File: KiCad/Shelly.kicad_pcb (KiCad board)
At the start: 2 copper layers, 15 x 30 mm, 15 parts, among them J1 Shelly 1, J2 Shelly 2, J3 Shelly i3, J4 USB-C, U1 FT231XQ, U2 G3VM-61VY3(TR)

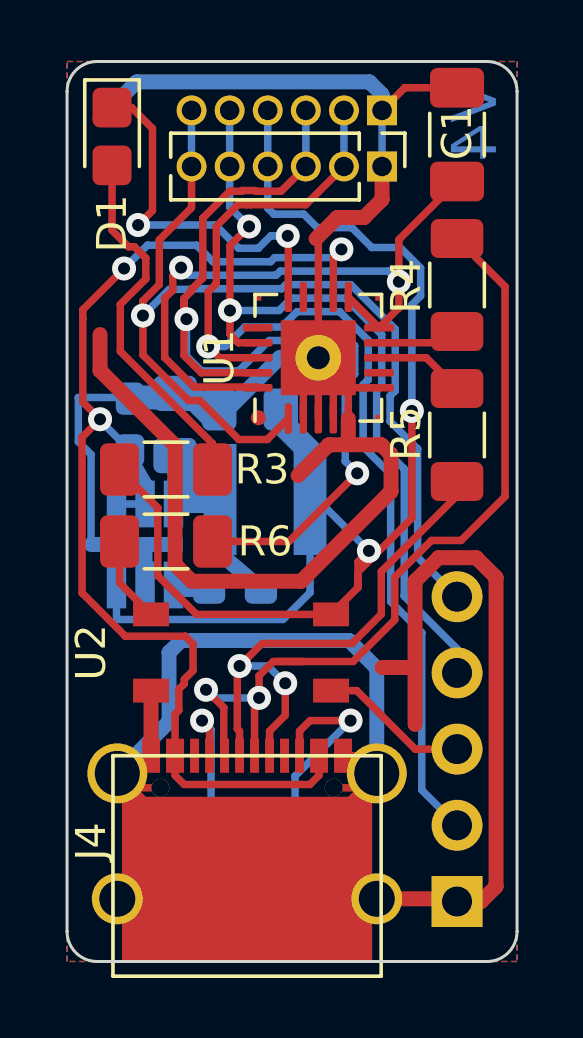
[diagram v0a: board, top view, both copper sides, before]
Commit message: Regulator
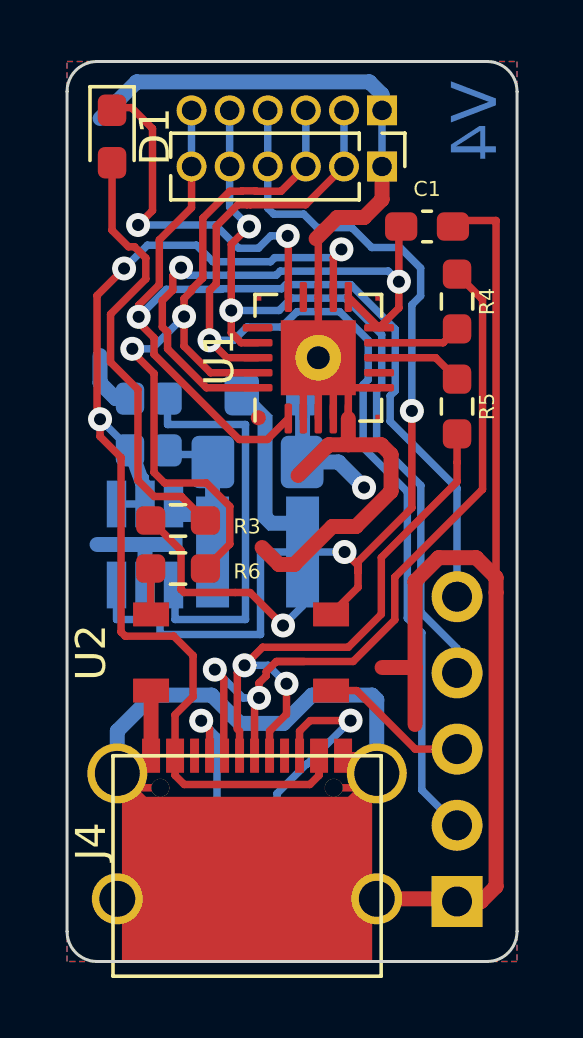
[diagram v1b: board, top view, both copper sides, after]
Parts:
- C1: footprint Capacitor_SMD:C_1206_3216Metric_Pad1.33x1.80mm_HandSolder -> Capacitor_SMD:C_0603_1608Metric_Pad1.08x0.95mm_HandSolder
- D1: footprint LED_SMD:LED_0805_2012Metric_Castellated -> LED_SMD:LED_0603_1608Metric_Pad1.05x0.95mm_HandSolder
- R1, R2, R3, R4, R5, R6: footprint Resistor_SMD:R_1206_3216Metric_Pad1.30x1.75mm_HandSolder -> Resistor_SMD:R_0603_1608Metric_Pad0.98x0.95mm_HandSolder
- moved C1 3.22 mm to (182.0, 64.5), turned to 0 degrees
- moved R3 1.75 mm to (173.7, 74.3)
- moved R6 0.98 mm to (173.7, 75.9)
- moved R5 0.95 mm to (183.0, 70.5)
- moved R2 0.60 mm to (177.0, 86.0)
- moved R4 0.55 mm to (183.0, 67.0)
- moved R1 0.21 mm to (175.0, 86.0)
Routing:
- net GND: track 143.9 -> 132.8 mm, vias 0 -> 1
- net RST: track 32.6 -> 25.4 mm
- net Net-(C1-Pad1): track 21.7 -> 19.3 mm
- net Net-(D1-Pad2): track 12.3 -> 14.8 mm
- net Net-(J4-PadA7): track 28.7 -> 26.8 mm
- net Net-(J4-PadA6): track 18.4 -> 19.8 mm
- net Net-(R6-Pad1): track 2.86 -> 1.54 mm
- net VBUS: track 40.7 -> 39.6 mm
- net Net-(J4-PadB5): track 6.86 -> 7.81 mm
- net Net-(J4-PadA5): track 4.83 -> 5.61 mm
- net +3V3: track 39.8 -> 40.2 mm, vias 2 -> 3
